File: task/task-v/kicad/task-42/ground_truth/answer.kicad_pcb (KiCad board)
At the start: 3 copper layers, 60 x 60 mm, 0 parts

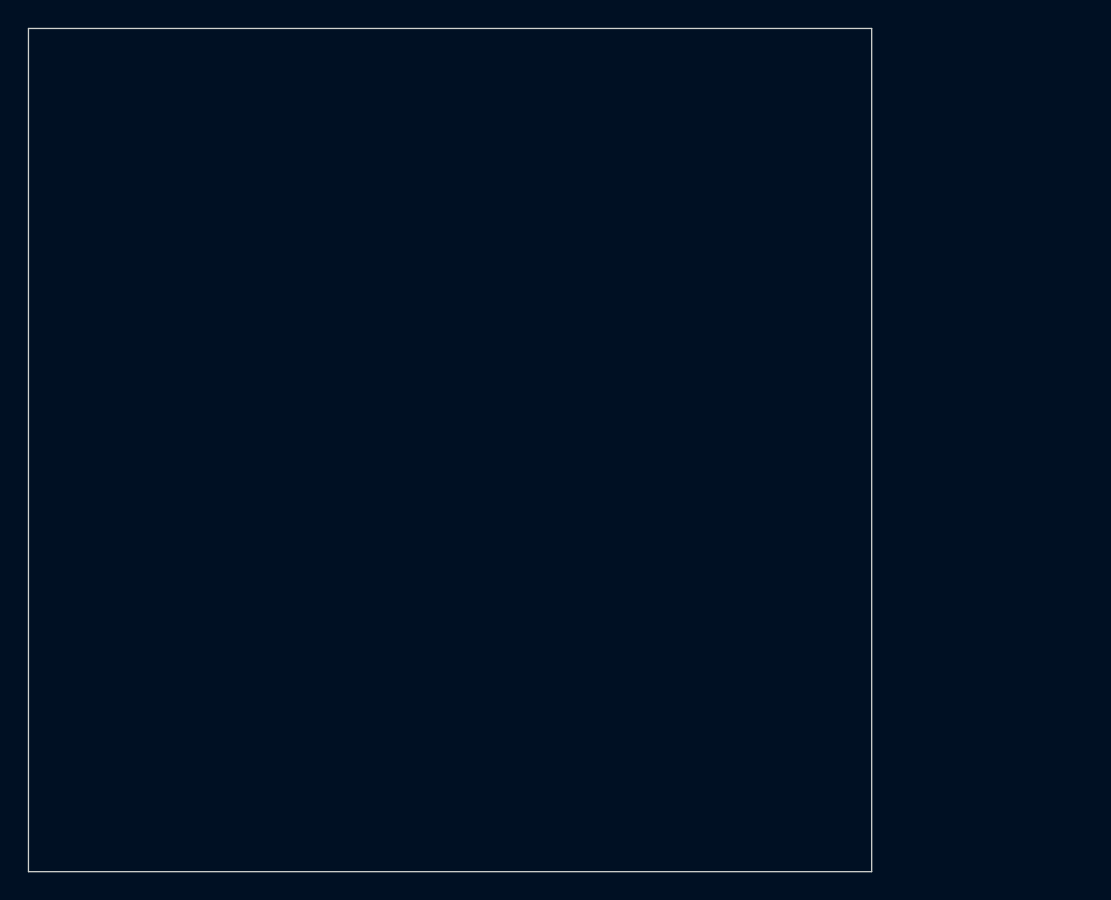
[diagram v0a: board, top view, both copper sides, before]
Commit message: Refine engineering task metadata and instructions
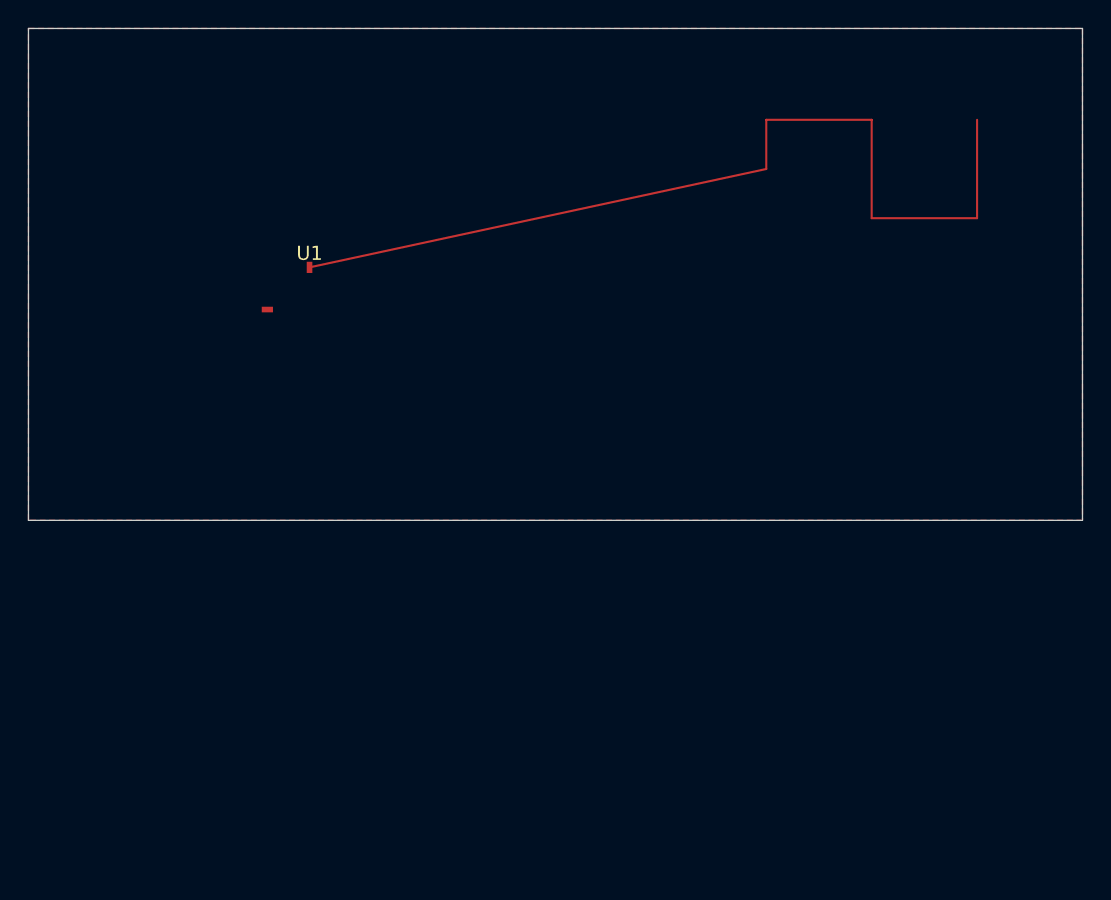
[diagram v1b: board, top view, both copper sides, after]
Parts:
- added U1: nRF52, Package_QFN:QFN-32_5x5mm_P0.5mm, F.Cu at (20.0, 20.0)
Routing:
- net RF_IN: track 0.00 -> 33.2 mm
- net ANT: track 0.00 -> 32.5 mm
- added copper zone on F.Cu, net GND
- removed copper zone on In1.Cu, net +3V3
- removed copper zone on In1.Cu, net GND
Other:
- board size 60 x 60 mm -> 75 x 35 mm
- copper layers 3 -> 2
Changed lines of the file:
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@@
   (layers
     (0 "F.Cu" signal)
-    (1 "In1.Cu" power)
     (31 "B.Cu" signal)
     (36 "B.SilkS" user "B.Silkscreen")
@@
   (net 0 "")
   (net 1 "GND")
-  (net 2 "+3V3")
+  (net 2 "ANT")
+  (net 3 "RF_IN")
+  (footprint "Package_QFN:QFN-32_5x5mm_P0.5mm"
+    (layer "F.Cu")
+    (at 20 20)
+    (property "Reference" "U1" (at 0 -4) (layer "F.SilkS") (effects (font (size 1 1) (thickness 0.15))))
+    (property "Value" "nRF52" (at 0 4) (layer "F.Fab") (effects (font (size 1 1) (thickness 0.15))))
+    (pad "1" smd rect (at 0 -3) (size 0.4 0.8) (layers "F.Cu" "F.Paste" "F.Mask") (net 3 "RF_IN"))
+    (pad "2" smd rect (at -3 0) (size 0.8 0.4) (layers "F.Cu" "F.Paste" "F.Mask") (net 1 "GND"))
+  )
+  (segment (start 20 17) (end 52.5 10) (width 0.15) (layer "F.Cu") (net 3))
+  (segment (start 52.5 10) (end 52.5 6.5) (width 0.15) (layer "F.Cu") (net 2))
+  (segment (start 52.5 6.5) (end 60 6.5) (width 0.15) (layer "F.Cu") (net 2))
+  (segment (start 60 6.5) (end 60 13.5) (width 0.15) (layer "F.Cu") (net 2))
+  (segment (start 60 13.5) (end 67.5 13.5) (width 0.15) (layer "F.Cu") (net 2))
+  (segment (start 67.5 13.5) (end 67.5 6.5) (width 0.15) (layer "F.Cu") (net 2))
   (zone
     (net 1)
     (net_name "GND")
-    (layer "In1.Cu")
-    (name "GND_PLANE")
-    (priority 0)
+    (layer "F.Cu")
+    (name "GND_TOP")
     (hatch edge 0.508)
     (connect_pads (clearance 0.5))
     (min_thickness 0.25)
     (fill yes (thermal_gap 0.5) (thermal_bridge_width 0.5))
-    (polygon (pts (xy 0 0) (xy 60 0) (xy 60 60) (xy 0 60)))
+    (polygon (pts (xy 0 0) (xy 75 0) (xy 75 35) (xy 0 35)))
   )
+  (gr_rect (start 0 0) (end 75 35) (layer "Edge.Cuts") (width 0.05))
   (zone
-    (net 2)
-    (net_name "+3V3")
-    (layer "In1.Cu")
-    (name "V33_ZONE")
-    (priority 10)
-    (hatch edge 0.508)
-    (connect_pads (clearance 0.5))
-    (min_thickness 0.25)
-    (fill yes (thermal_gap 0.5) (thermal_bridge_width 0.5))
-    (polygon (pts (xy 0 0) (xy 30 0) (xy 30 30) (xy 0 30)))
+    (layer "F.Cu")
+    (name "ANT_KEEPOUT")
+    (hatch none 0.508)
+    (keepout (tracks not_allowed) (vias not_allowed) (pads not_allowed) (copperpour not_allowed) (footprints allowed))
+    (polygon (pts (xy 52.5 6.5) (xy 67.5 6.5) (xy 67.5 13.5) (xy 52.5 13.5)))
   )
-  (gr_rect (start 0 0) (end 60 60) (layer "Edge.Cuts") (width 0.05))
 )
